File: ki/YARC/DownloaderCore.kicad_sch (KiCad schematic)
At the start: 13 parts, among them J1 NANOIO_EXT, J2 MCR_EXT, J3 PULSE_EXT, U1 74HCT574, U2 74HCT574, U3 74HCT574, U4 74HCT574, U5 74HCT574, U6 74LS138, U7 74HCT574, U8 74HC245, U9 74LS138

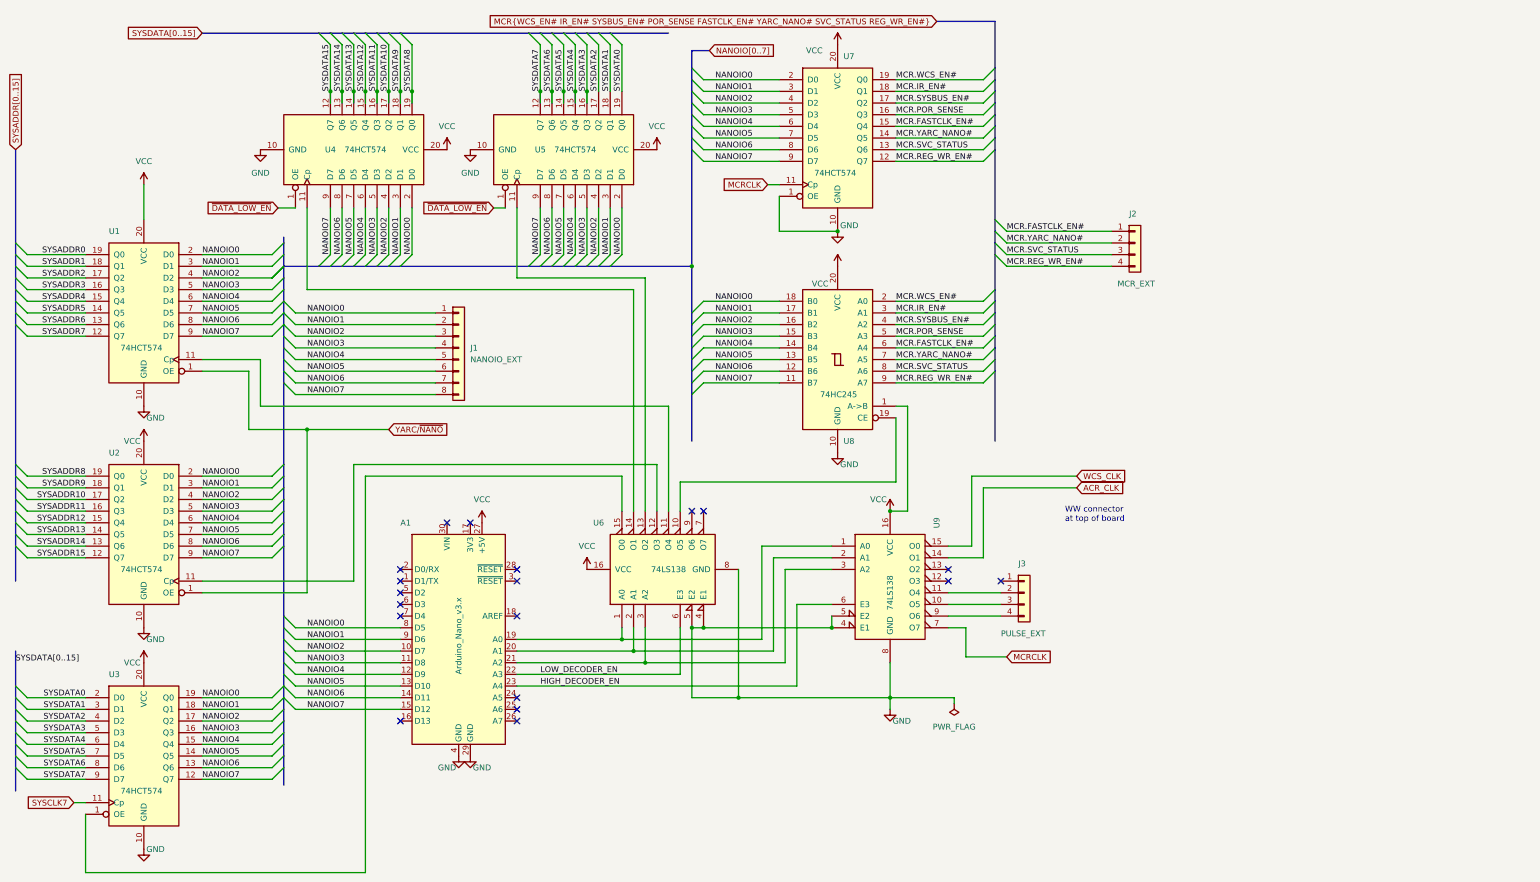
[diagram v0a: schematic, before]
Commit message: Continuing cleanup of schematic
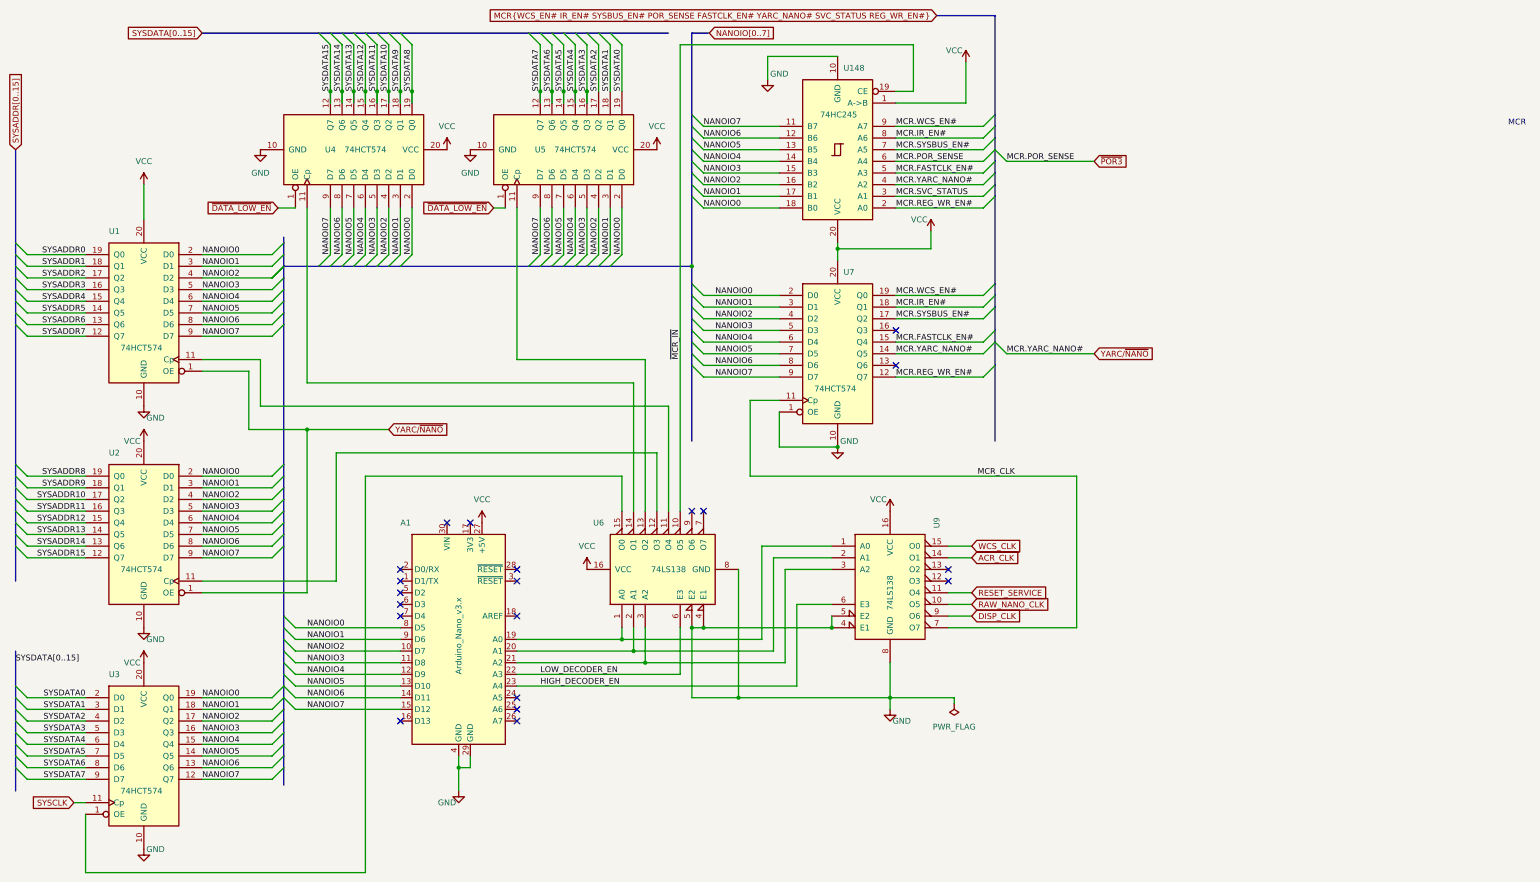
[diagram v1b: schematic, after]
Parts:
- removed J1: NANOIO_EXT, symbol Connector_Generic:Conn_01x08
- removed J2: MCR_EXT, symbol Connector_Generic:Conn_01x04
- removed J3: PULSE_EXT, symbol Connector_Generic:Conn_01x04
- removed U8: 74HC245, symbol 74xx:74HC245
- added U148: 74HC245, symbol 74xx:74HC245
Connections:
- net MCR.YARC_NANO# is gone; now on net YARC/~{NANO}: U7.14 (Q5)
- net GND: now also U148.10 (GND)
- net MCR.FASTCLK_EN#: now also U148.5 (A3)
- net MCR.IR_EN#: now also U148.8 (A6)
- net MCR.REG_WR_EN#: now also U148.2 (A0)
- net MCR.SVC_STATUS: now also U148.3 (A1); no longer U7.13 (Q6)
- net MCR.SYSBUS_EN#: now also U148.7 (A5)
- net MCR.WCS_EN#: now also U148.9 (A7)
- net NANOIO0: now also U148.18 (B0)
- net NANOIO1: now also U148.17 (B1)
- net NANOIO2: now also U148.16 (B2)
- net NANOIO3: now also U148.15 (B3)
- net NANOIO4: now also U148.14 (B4)
- net NANOIO5: now also U148.13 (B5)
- net NANOIO6: now also U148.12 (B6)
- net NANOIO7: now also U148.11 (B7)
- net VCC: now also U148.1 (A->B), U148.20 (VCC)
- net YARC/~{NANO}: now also U148.4 (A2)
- net ~{MCR_IN}: now reaches U6.10 (O5)
- net ~{MCR_IN}: now also U148.19 (CE)
- net RESET_SERVICE: now reaches U9.11 (O4)
- net RAW_NANO_CLK: now reaches U9.10 (O5)
- net DISP_CLK: now reaches U9.9 (O6)
- net MCR.POR_SENSE: no longer names the net of U7.16 (Q3)
- net MCRCLK renamed MCR_CLK
- net SYSCLK7 renamed SYSCLK
- new net ~{POR3}: U148.6 (A4)
- no-connect marks 19 -> 20
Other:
- note added: "MCR"
- note removed: "WW connector at top of board"
- moved on the sheet: U7

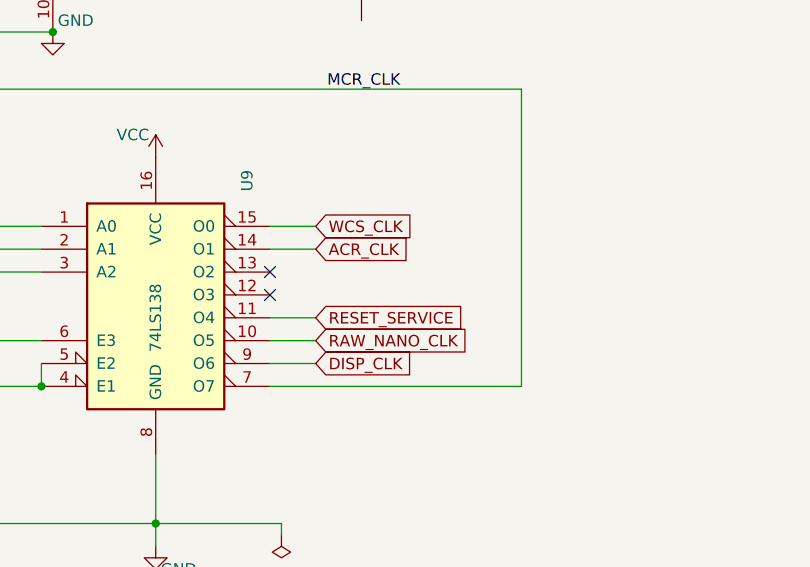
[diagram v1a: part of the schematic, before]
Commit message: Ongoing schematic changes
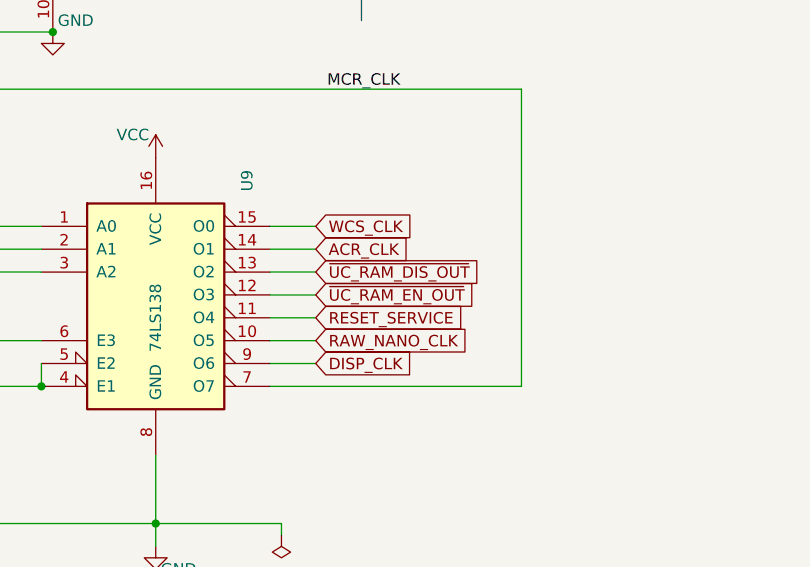
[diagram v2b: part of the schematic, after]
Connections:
- net ~{UC_RAM_EN_OUT}: now reaches U9.12 (O3)
- net ~{UC_RAM_DIS_OUT}: now reaches U9.13 (O2)
- no-connect marks 20 -> 18
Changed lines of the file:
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@@
   (no_connect (at 114.3 124.46))
   (no_connect (at 124.46 134.62))
-  (no_connect (at 218.44 134.62))
   (no_connect (at 109.22 124.46))
   (no_connect (at 165.1 121.92))
   (no_connect (at 124.46 165.1))
   (no_connect (at 99.06 139.7))
-  (no_connect (at 218.44 137.16))
   (no_connect (at 124.46 167.64))
   (no_connect (at 99.06 142.24))
@@
     (stroke (width 0) (type default))
   )
+  (wire (pts (xy 218.44 137.16) (xy 223.52 137.16))
+    (stroke (width 0) (type default))
+  )
   (wire (pts (xy 76.2 157.48) (xy 99.06 157.48))
     (stroke (width 0) (type default))
@@
     (stroke (width 0) (type default))
   )
+  (wire (pts (xy 218.44 134.62) (xy 223.52 134.62))
+    (stroke (width 0) (type default))
+  )
   (bus (pts (xy 162.56 38.1) (xy 162.56 40.64))
     (stroke (width 0) (type default))
@@
     (effects (font (size 1.27 1.27)) (justify left bottom))
   )
-  (label "NANOIO7" (at 165.1 38.1 0)
+  (label "NANOIO7" (at 165.1 38.1 0) (fields_autoplaced)
     (effects (font (size 1.27 1.27)) (justify left bottom))
   )
@@
     (effects (font (size 1.27 1.27)) (justify left bottom))
   )
-  (label "NANOIO3" (at 165.1 48.26 0)
+  (label "NANOIO3" (at 165.1 48.26 0) (fields_autoplaced)
     (effects (font (size 1.27 1.27)) (justify left bottom))
   )
@@
     (effects (font (size 1.27 1.27)) (justify left bottom))
   )
-  (label "MCR.POR_SENSE" (at 231.14 45.72 0)
+  (label "MCR.POR_SENSE" (at 231.14 45.72 0) (fields_autoplaced)
     (effects (font (size 1.27 1.27)) (justify left bottom))
   )
@@
     (effects (font (size 1.27 1.27)) (justify right bottom))
   )
-  (label "NANOIO5" (at 165.1 43.18 0)
+  (label "NANOIO5" (at 165.1 43.18 0) (fields_autoplaced)
     (effects (font (size 1.27 1.27)) (justify left bottom))
   )
@@
     (effects (font (size 1.27 1.27)) (justify left bottom))
   )
-  (label "MCR.SYSBUS_EN#" (at 207.01 43.18 0)
+  (label "MCR.SYSBUS_EN#" (at 207.01 43.18 0) (fields_autoplaced)
     (effects (font (size 1.27 1.27)) (justify left bottom))
   )
@@
     (effects (font (size 1.27 1.27)) (justify left bottom))
   )
-  (label "NANOIO4" (at 165.1 45.72 0)
+  (label "NANOIO4" (at 165.1 45.72 0) (fields_autoplaced)
     (effects (font (size 1.27 1.27)) (justify left bottom))
   )
@@
     (effects (font (size 1.27 1.27)) (justify left bottom))
   )
-  (label "MCR.REG_WR_EN#" (at 207.01 55.88 0)
+  (label "MCR.REG_WR_EN#" (at 207.01 55.88 0) (fields_autoplaced)
     (effects (font (size 1.27 1.27)) (justify left bottom))
   )
@@
     (effects (font (size 1.27 1.27)) (justify left bottom))
   )
-  (label "MCR.POR_SENSE" (at 207.01 45.72 0)
+  (label "MCR.POR_SENSE" (at 207.01 45.72 0) (fields_autoplaced)
     (effects (font (size 1.27 1.27)) (justify left bottom))
   )
@@
     (effects (font (size 1.27 1.27)) (justify left bottom))
   )
-  (label "NANOIO1" (at 165.1 53.34 0)
-    (effects (font (size 1.27 1.27)) (justify left bottom))
-  )
-  (label "NANOIO0" (at 165.1 55.88 0)
+  (label "NANOIO1" (at 165.1 53.34 0) (fields_autoplaced)
+    (effects (font (size 1.27 1.27)) (justify left bottom))
+  )
+  (label "NANOIO0" (at 165.1 55.88 0) (fields_autoplaced)
     (effects (font (size 1.27 1.27)) (justify left bottom))
   )
@@
     (effects (font (size 1.27 1.27)) (justify left bottom))
   )
-  (label "NANOIO6" (at 165.1 40.64 0)
+  (label "NANOIO6" (at 165.1 40.64 0) (fields_autoplaced)
     (effects (font (size 1.27 1.27)) (justify left bottom))
   )
@@
     (effects (font (size 1.27 1.27)) (justify right bottom))
   )
-  (label "MCR.YARC_NANO#" (at 231.14 87.63 0)
-    (effects (font (size 1.27 1.27)) (justify left bottom))
-  )
-  (label "NANOIO2" (at 165.1 50.8 0)
+  (label "MCR.YARC_NANO#" (at 231.14 87.63 0) (fields_autoplaced)
+    (effects (font (size 1.27 1.27)) (justify left bottom))
+  )
+  (label "NANOIO2" (at 165.1 50.8 0) (fields_autoplaced)
     (effects (font (size 1.27 1.27)) (justify left bottom))
   )
@@
     (effects (font (size 1.27 1.27)) (justify right bottom))
   )
-  (label "MCR.SVC_STATUS" (at 207.01 53.34 0)
+  (label "MCR.SVC_STATUS" (at 207.01 53.34 0) (fields_autoplaced)
     (effects (font (size 1.27 1.27)) (justify left bottom))
   )
@@
     (effects (font (size 1.27 1.27)) (justify left bottom))
   )
-  (label "MCR.IR_EN#" (at 207.01 40.64 0)
+  (label "MCR.IR_EN#" (at 207.01 40.64 0) (fields_autoplaced)
     (effects (font (size 1.27 1.27)) (justify left bottom))
   )
@@
     (effects (font (size 1.27 1.27)) (justify left bottom))
   )
-  (label "MCR.YARC_NANO#" (at 207.01 50.8 0)
+  (label "MCR.YARC_NANO#" (at 207.01 50.8 0) (fields_autoplaced)
     (effects (font (size 1.27 1.27)) (justify left bottom))
   )
@@
     (effects (font (size 1.27 1.27)) (justify right bottom))
   )
-  (label "MCR.WCS_EN#" (at 207.01 38.1 0)
+  (label "MCR.WCS_EN#" (at 207.01 38.1 0) (fields_autoplaced)
     (effects (font (size 1.27 1.27)) (justify left bottom))
   )
@@
     (effects (font (size 1.27 1.27)) (justify left bottom))
   )
-  (label "MCR.FASTCLK_EN#" (at 207.01 48.26 0)
+  (label "MCR.FASTCLK_EN#" (at 207.01 48.26 0) (fields_autoplaced)
     (effects (font (size 1.27 1.27)) (justify left bottom))
   )
@@
     )
   )
+  (global_label "~{UC_RAM_EN_OUT}" (shape input) (at 223.52 137.16 0) (fields_autoplaced)
+    (effects (font (size 1.27 1.27)) (justify left))
+    (property "Intersheetrefs" "${INTERSHEET_REFS}" (at 241.3545 137.0806 0)
+      (effects (font (size 1.27 1.27)) (justify left) hide)
+    )
+  )
   (global_label "SYSADDR[0..15]" (shape input) (at 15.24 43.18 90) (fields_autoplaced)
     (effects (font (size 1.27 1.27)) (justify left))
@@
       (effects (font (size 1.27 1.27)) (justify left) hide)
     )
+  )
+  (global_label "~{UC_RAM_DIS_OUT}" (shape input) (at 223.52 134.62 0) (fields_autoplaced)
+    (effects (font (size 1.27 1.27)) (justify left))
+    (property "Intersheetrefs" "${INTERSHEET_REFS}" (at 241.9593 134.5406 0)
+      (effects (font (size 1.27 1.27)) (justify left) hide)
+    )
